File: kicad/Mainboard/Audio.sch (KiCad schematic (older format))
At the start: 72 parts, among them J10 MIC_EXT, J12 SPK_EXT, Q4 BSS138, Q5 BSS138, SW1 INT_PTT_SW, U10 LM386, U8 HEF4066B, U9 OPA340UA

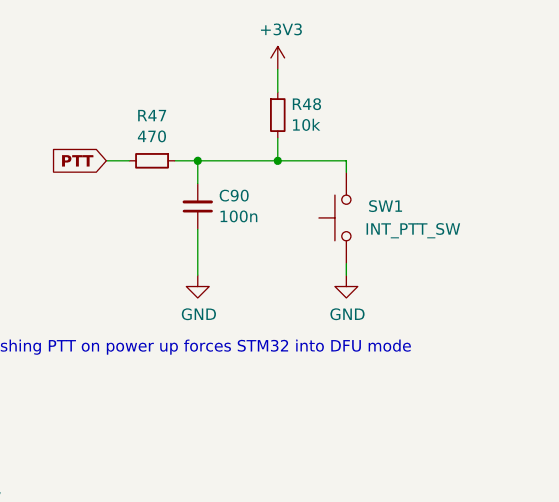
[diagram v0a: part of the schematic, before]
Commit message: Update
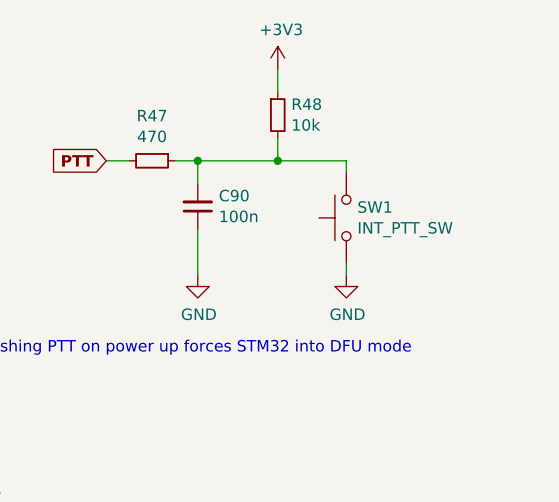
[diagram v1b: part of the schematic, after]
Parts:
- removed SW1: INT_PTT_SW, Button_Switch_THT:SW_Tactile_SKHH_Angled, symbol Mainboard-rescue:SW_Push-switches
- added SW1: INT_PTT_SW, Button_Switch_SMD:SW_Push_1P1T_NO_CK_KMR2, symbol Switch:SW_Push
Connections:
- net GND: now also SW1.1
- net at C90.2, R47.1, R48.2: now also SW1.2
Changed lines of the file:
@@
-$EndComp
-$Comp
-L Mainboard-rescue:SW_Push-switches SW1
-U 1 1 5DFE1B21
-P 10500 1650
-F 0 "SW1" V 10450 1400 50  0000 L CNN
-F 1 "INT_PTT_SW" V 10550 1150 50  0000 L CNN
-F 2 "Button_Switch_THT:SW_Tactile_SKHH_Angled" H 10500 1850 50  0001 C CNN
-F 3 "" H 10500 1850 50  0001 C CNN
-	1    10500 1650
-	0    -1   1    0
 $EndComp
 $Comp
@@
 	4550 1500 4650 1500
 Wire Wire Line
-	10500 1850 10500 1900
-Wire Wire Line
 	10500 1450 10500 1400
 Wire Wire Line
@@
 Wire Wire Line
 	3500 6100 3650 6100
+$Comp
+L Switch:SW_Push SW1
+U 1 1 6121661D
+P 10500 1650
+F 0 "SW1" V 10546 1602 50  0000 R CNN
+F 1 "INT_PTT_SW" V 10455 1602 50  0000 R CNN
+F 2 "Button_Switch_SMD:SW_Push_1P1T_NO_CK_KMR2" H 10500 1850 50  0001 C CNN
+F 3 "~" H 10500 1850 50  0001 C CNN
+	1    10500 1650
+	0    -1   -1   0
+$EndComp
+Wire Wire Line
+	10500 1850 10500 1900
 $EndSCHEMATC
